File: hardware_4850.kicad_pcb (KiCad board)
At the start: 2 copper layers, 207.2 x 123 mm, 283 parts, among them J101 PWM, J102 ADC, J103 PWM, J104 ADC, J105 +, J106 A, J107 B, J108 C, J109 GND, J1101 HALL, J1102 PWM_EN, J1103 CAN_IN, J1104 CAN_Out, J501 Enable, J601 AIN, J602 USB_B_Mini, J701 MOT_TEMP, P1101 SWD, Q201 NCEP6080AG, Q202 NCEP6080AG, Q203 NCEP6080AG, Q204 NCEP6080AG, Q301 NCEP6080AG, Q302 NCEP6080AG, Q303 NCEP6080AG, Q304 NCEP6080AG, Q401 NCEP6080AG, Q402 NCEP6080AG, Q403 NCEP6080AG, Q404 NCEP6080AG, U1001 GS8632-MR, U1101 TCAN334, U1102 24LC04, U1103 AP2204K-5.0, U201 LM5109BMA, U202 INA240A1PWR, U301 LM5109BMA, U302 INA240A1PWR, U401 LM5109BMA, U402 INA240A1PWR, U501 LMR12010Y, U502 LM5008, U601 STM32F730R8Tx, U701 GS8632-MR, U801 GS8632-MR, U901 GS8632-MR, X601 SM44T

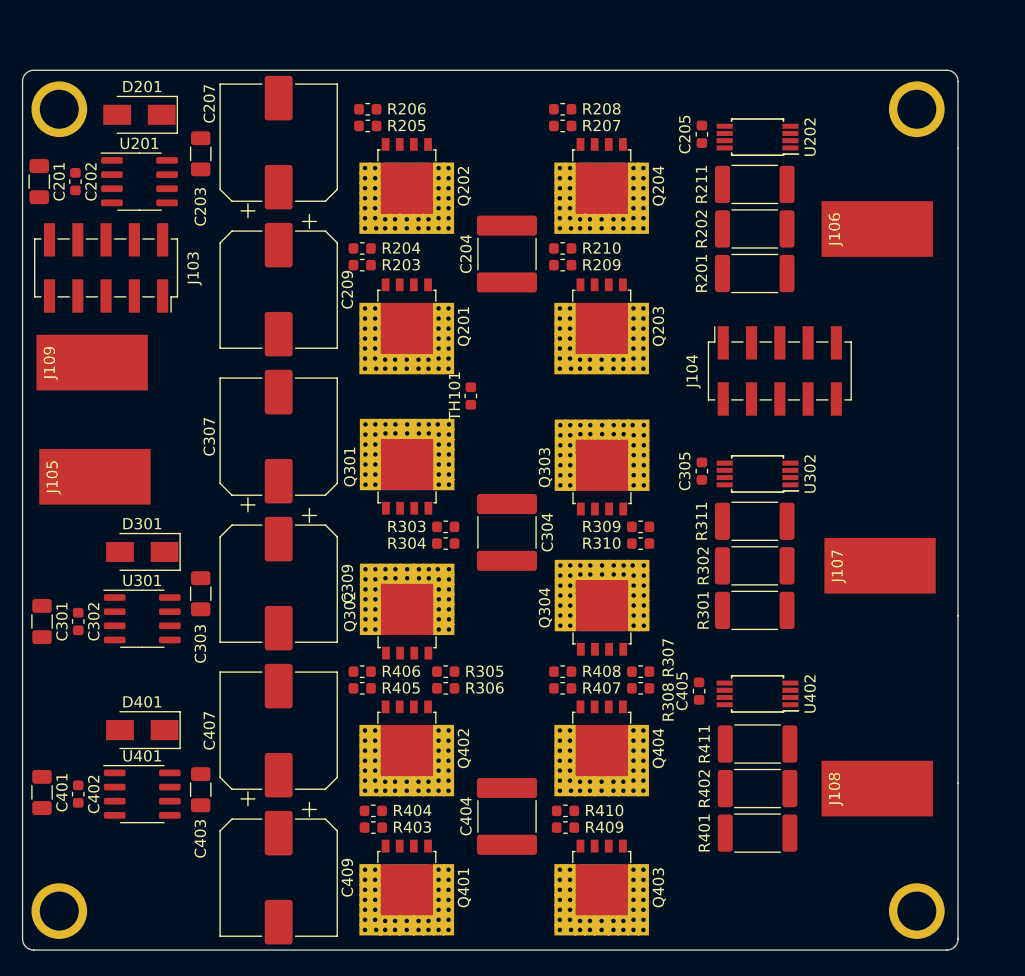
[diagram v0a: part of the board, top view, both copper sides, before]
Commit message: started routing of power stage
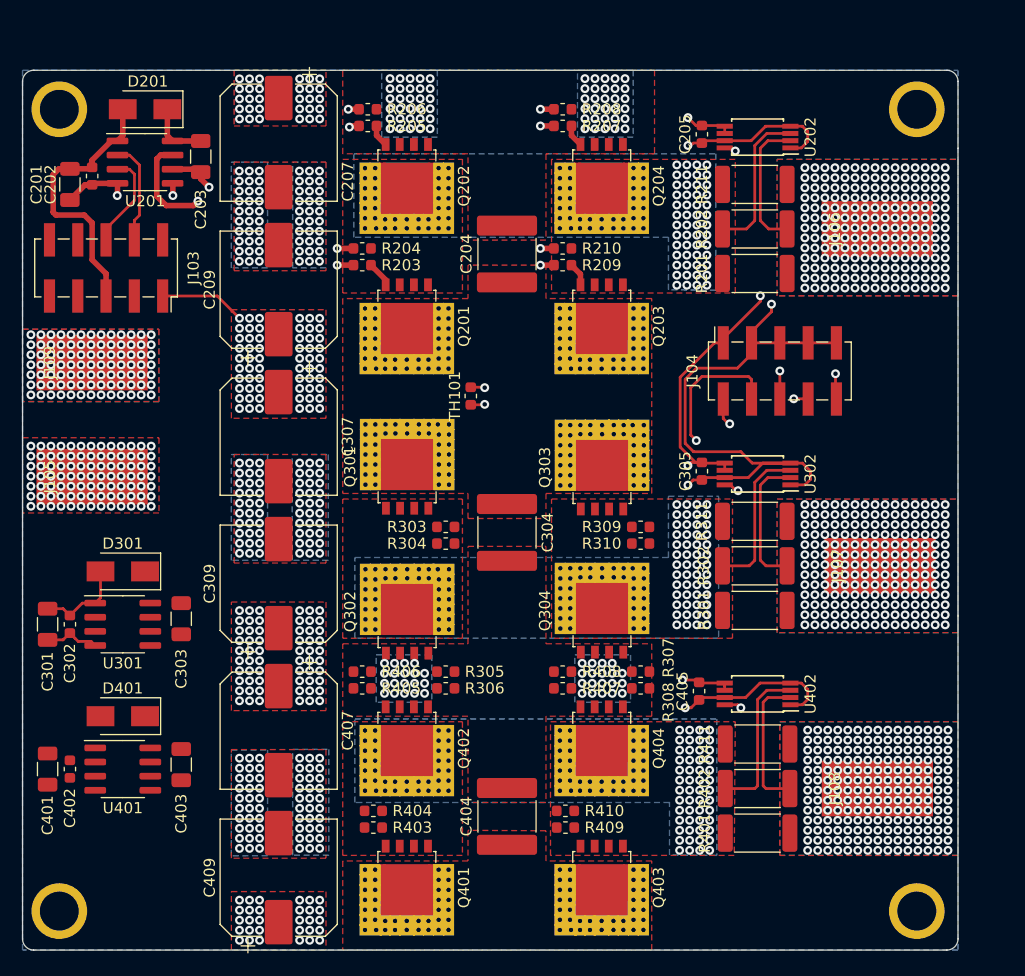
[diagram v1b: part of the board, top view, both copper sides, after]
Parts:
- moved C303 2.85 mm to (71.2, 152.2)
- moved C403 2.85 mm to (71.2, 165.3)
- moved U401 2.85 mm to (66.0, 165.8)
- moved C201 2.76 mm to (61.2, 113.2)
- moved D301 2.47 mm to (66.0, 148.0)
- moved C402 2.37 mm to (61.2, 165.8)
- moved C401 2.16 mm to (59.2, 165.8)
- moved D401 2.15 mm to (66.0, 161.0)
- moved U201 1.82 mm to (68.0, 111.2)
- moved U301 1.82 mm to (66.0, 152.8)
- moved C202 1.58 mm to (63.2, 112.5)
- moved C302 0.79 mm to (61.2, 152.8)
- moved D201 0.71 mm to (68.0, 106.5)
- moved C301 0.56 mm to (59.2, 152.8)
- moved Q304 0.25 mm to (109.0, 152.4)
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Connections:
- R203 pad 2: Net-(C203-Pad2) -> Net-(R203-Pad2)
- R209 pad 2: Net-(C203-Pad2) -> Net-(R203-Pad2)
- R303 pad 2: Net-(C303-Pad2) -> Net-(R303-Pad2)
- R309 pad 2: Net-(C303-Pad2) -> Net-(R303-Pad2)
- R403 pad 2: Net-(C403-Pad2) -> Net-(R403-Pad2)
- R409 pad 2: Net-(C403-Pad2) -> Net-(R403-Pad2)
- U201 pad 7: Net-(C203-Pad2) -> Net-(R203-Pad2)
- U301 pad 7: Net-(C303-Pad2) -> Net-(R303-Pad2)
- U401 pad 7: Net-(C403-Pad2) -> Net-(R403-Pad2)
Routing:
- net GND: track 0.00 -> 135.0 mm, vias 0 -> 4
- net +3.3VA: track 0.00 -> 79.4 mm, vias 0 -> 4
- net Net-(C201-Pad2): track 0.00 -> 52.0 mm, vias 0 -> 3
- net Net-(R205-Pad2): track 0.00 -> 40.4 mm, vias 0 -> 3
- net Net-(J104-Pad10): track 0.00 -> 35.6 mm, vias 0 -> 2
- net +12P: track 0.00 -> 32.8 mm
- net Net-(J104-Pad8): track 0.00 -> 30.9 mm, vias 0 -> 2
- net /phase_c/I: track 0.00 -> 30.8 mm, vias 0 -> 2
- net Net-(R203-Pad2): track 0.00 -> 30.0 mm, vias 0 -> 3
- net Net-(C203-Pad2): track 0.00 -> 25.2 mm, vias 0 -> 3
- net /phase_a/I: track 0.00 -> 25.0 mm, vias 0 -> 2
- net /phase_b/I: track 0.00 -> 20.2 mm, vias 0 -> 2
- net Net-(Q401-Pad1): track 0.00 -> 14.0 mm, vias 0 -> 52
- net Net-(Q301-Pad1): track 0.00 -> 13.8 mm, vias 0 -> 52
- net Net-(Q201-Pad1): track 0.00 -> 13.6 mm, vias 0 -> 52
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- added copper zone on B.Cu, net +BATT
- added copper zone on F.Cu, net +BATT
- added copper zone on GND, net +BATT
- added copper zone on B.Cu, net /phase_a/Phase
- added copper zone on F.Cu, net /phase_a/Phase
- added copper zone on B.Cu, net /phase_b/Phase
- added copper zone on F.Cu, net /phase_b/Phase
- added copper zone on B.Cu, net /phase_c/Phase
- added copper zone on F.Cu, net /phase_c/Phase
- added copper zone on B.Cu, net GNDPWR
- added copper zone on F.Cu, net GNDPWR
- added copper zone on GND, net GNDPWR
- added copper zone on B.Cu, net Net-(Q201-Pad1)
- added copper zone on F.Cu, net Net-(Q201-Pad1)
- added copper zone on B.Cu, net Net-(Q301-Pad1)
- added copper zone on F.Cu, net Net-(Q301-Pad1)
- added copper zone on B.Cu, net Net-(Q401-Pad1)
- added copper zone on F.Cu, net Net-(Q401-Pad1)
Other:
- copper layers 2 -> 4
- net class GateDrive added: clearance 0.2, trace_width 0.5, via_dia 0.8, via_drill 0.4
